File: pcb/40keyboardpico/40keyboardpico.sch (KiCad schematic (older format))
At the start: 44 parts, among them J1 Conn_01x04, J10 Conn_01x04, J11 AudioJack4, J2 Conn_01x04, J3 Conn_01x04, J4 Conn_01x04, J5 Conn_01x04, J6 Conn_01x04, J7 Conn_01x04, J8 Conn_01x04, J9 Conn_01x04, SW1 SW_Push, SW10 SW_Push, SW11 SW_Push, SW12 SW_Push, SW13 SW_Push, SW14 SW_Push, SW15 SW_Push, SW16 SW_Push, SW2 SW_Push, SW3 SW_Push, SW4 SW_Push, SW5 SW_Push, SW6 SW_Push, SW7 SW_Push, SW8 SW_Push, SW9 SW_Push, U1 Pico

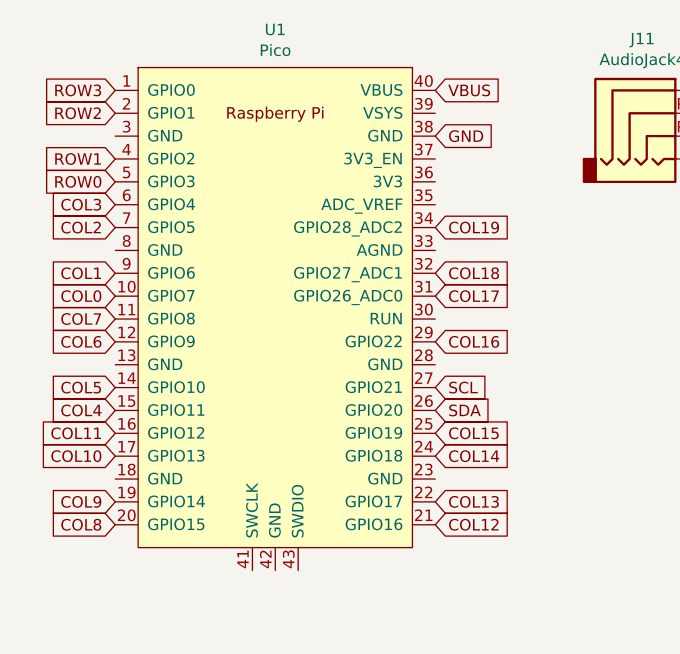
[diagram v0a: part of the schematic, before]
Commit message: Send it to all pcb.
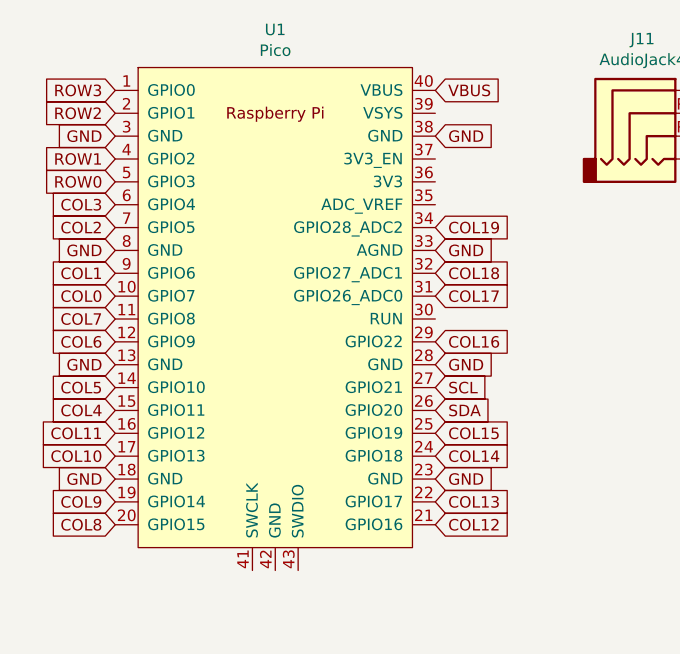
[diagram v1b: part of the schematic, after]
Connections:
- net GND: now also U1.13 (GND), U1.18 (GND), U1.23 (GND), U1.28 (GND), U1.3 (GND), U1.33 (AGND), U1.8 (GND)
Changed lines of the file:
@@
 Text GLabel 3200 1600 2    50   Input ~ 0
 COL19
+Text GLabel 3200 1700 2    50   Input ~ 0
+GND
+Text GLabel 3200 2200 2    50   Input ~ 0
+GND
+Text GLabel 3200 2700 2    50   Input ~ 0
+GND
+Text GLabel 1800 2700 0    50   Input ~ 0
+GND
+Text GLabel 1800 2200 0    50   Input ~ 0
+GND
+Text GLabel 1800 1700 0    50   Input ~ 0
+GND
+Text GLabel 1800 1200 0    50   Input ~ 0
+GND
 $EndSCHEMATC
